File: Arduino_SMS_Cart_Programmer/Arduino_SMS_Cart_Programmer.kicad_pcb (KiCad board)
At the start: 2 copper layers, 60.5 x 75.2 mm, 12 parts, among them J1 SEGA Master System Cartridge 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, U1 74HC595, U2 74HC595

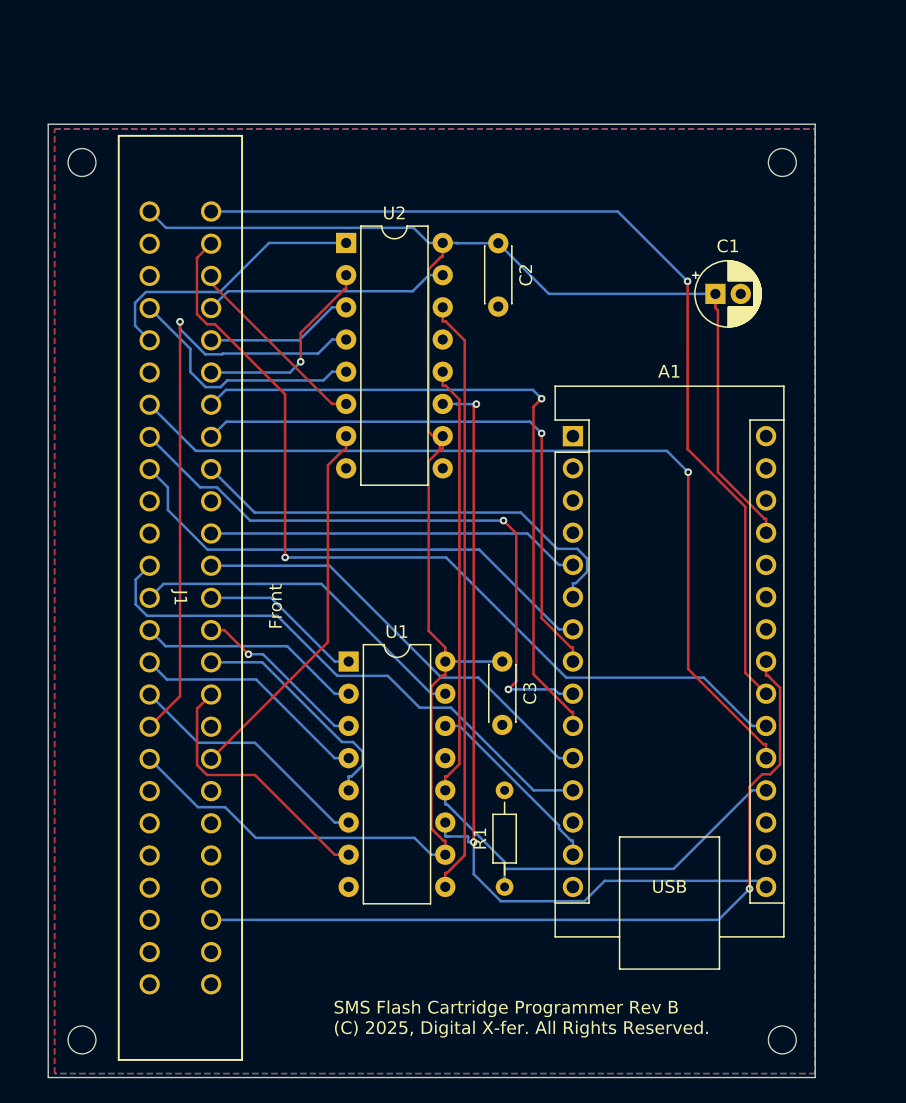
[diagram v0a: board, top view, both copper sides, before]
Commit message: Cleaned up RevB PCB.
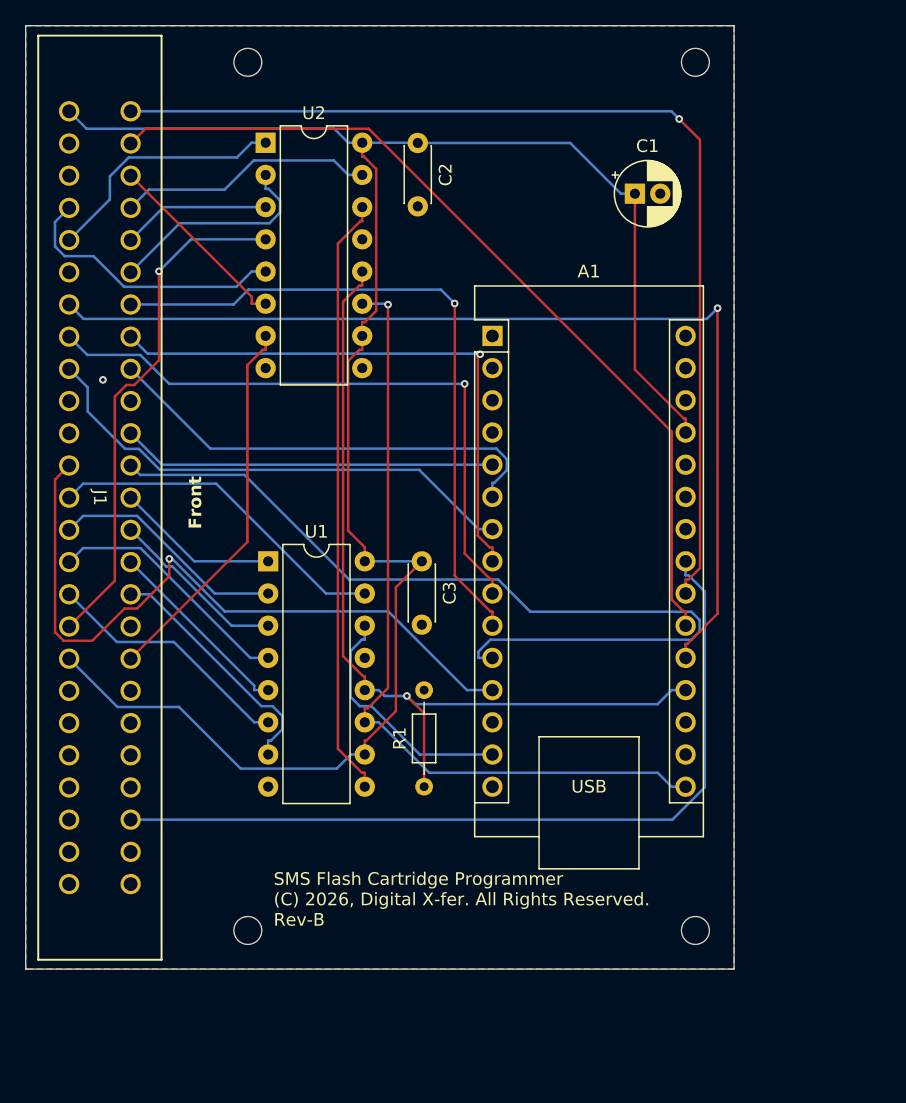
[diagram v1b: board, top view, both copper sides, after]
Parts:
- moved REF3 15.7 mm to (126.7, 124.7)
- moved REF1 15.3 mm to (126.7, 56.2)
- moved REF4 11.0 mm to (162.1, 124.7)
- moved REF2 10.5 mm to (162.1, 56.2)
- moved J1 10.1 mm to (124.0, 54.1)
- moved A1 10.1 mm to (146.0, 77.8)
- moved C1 10.1 mm to (157.3, 66.6)
- moved C3 10.1 mm to (140.5, 95.6)
- moved R1 10.1 mm to (140.7, 113.4)
- moved U1 10.1 mm to (128.3, 95.6)
- moved U2 10.1 mm to (128.2, 62.6)
- moved C2 10.1 mm to (140.2, 62.6)
- renumbered REF** to REF1, REF** to REF2, REF** to REF3, REF** to REF4
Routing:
- net D0: track 34.8 -> 70.5 mm
- net D1: track 44.1 -> 56.2 mm, vias 0 -> 1
- net /CE: track 69.9 -> 80.7 mm
- net /WR: track 75.0 -> 82.2 mm
- net A12: track 47.9 -> 40.8 mm
- net SCK: track 67.7 -> 63.3 mm, vias 2 -> 1
- net MOSI: track 15.1 -> 19.3 mm
- net A5: track 18.5 -> 15.2 mm
- net /RD: track 71.9 -> 68.9 mm, vias 1 -> 0
- net A9: track 22.0 -> 19.7 mm
- net A13: track 19.6 -> 21.9 mm
- net /RST: track 63.3 -> 64.9 mm, vias 1 -> 0
- net A10: track 15.8 -> 17.3 mm, vias 1 -> 0
- net RCLK: track 67.1 -> 68.5 mm, vias 0 -> 1
- net VCC: track 150.8 -> 152.2 mm
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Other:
- board size 60.5 x 75.2 mm -> 55.9 x 74.4 mm
- board text added: "SMS Flash Cartridge Programmer (C) 2026, Digital X-fer. All Rights Reserved. Rev-B"
- board text removed: "SMS Flash Cartridge Programmer Rev B (C) 2025, Digital X-fer. All Rights Reserved."
